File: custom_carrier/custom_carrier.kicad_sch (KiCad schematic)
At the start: 11 parts, among them J1 ERF5-040-05.0-X-DV, J13 PJ-002AH-SMT-TR, J14 87832-1420, J2 ERF5-040-05.0-X-DV, J3 ERF5-040-05.0-X-DV, J4 ERF5-040-05.0-X-DV, J5 45230-220230, J6 45230-220230

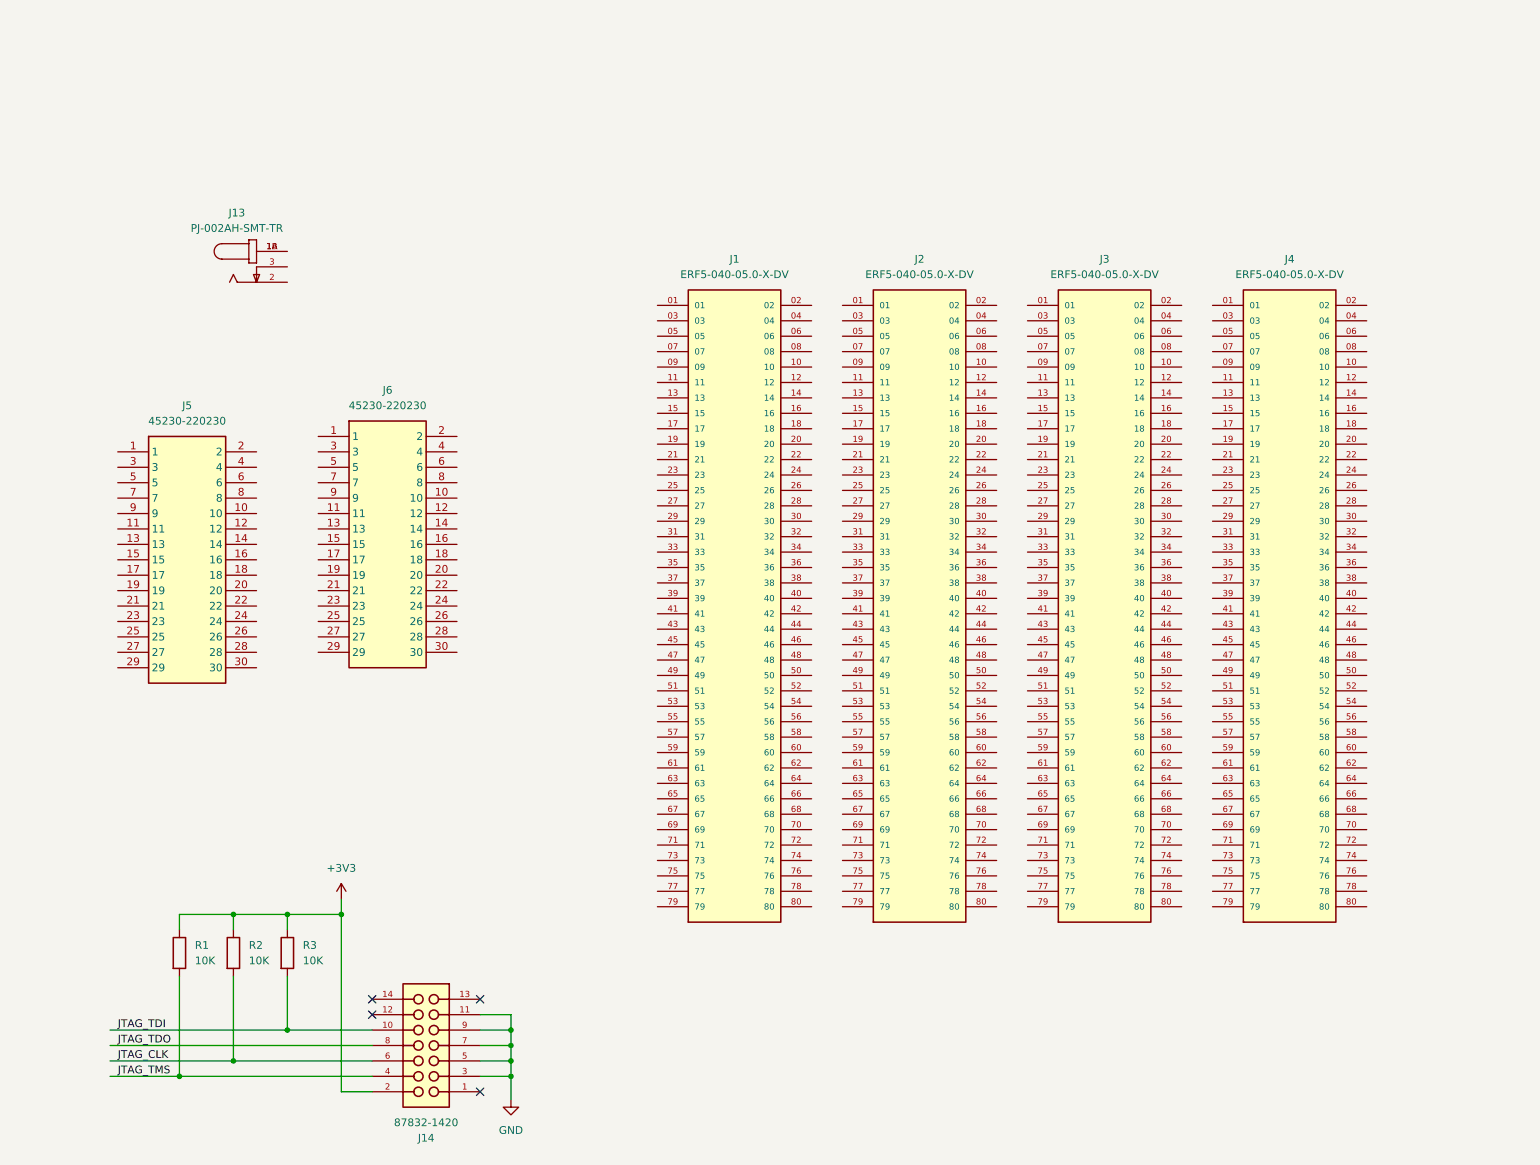
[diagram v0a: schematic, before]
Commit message: working on high-speed cables.
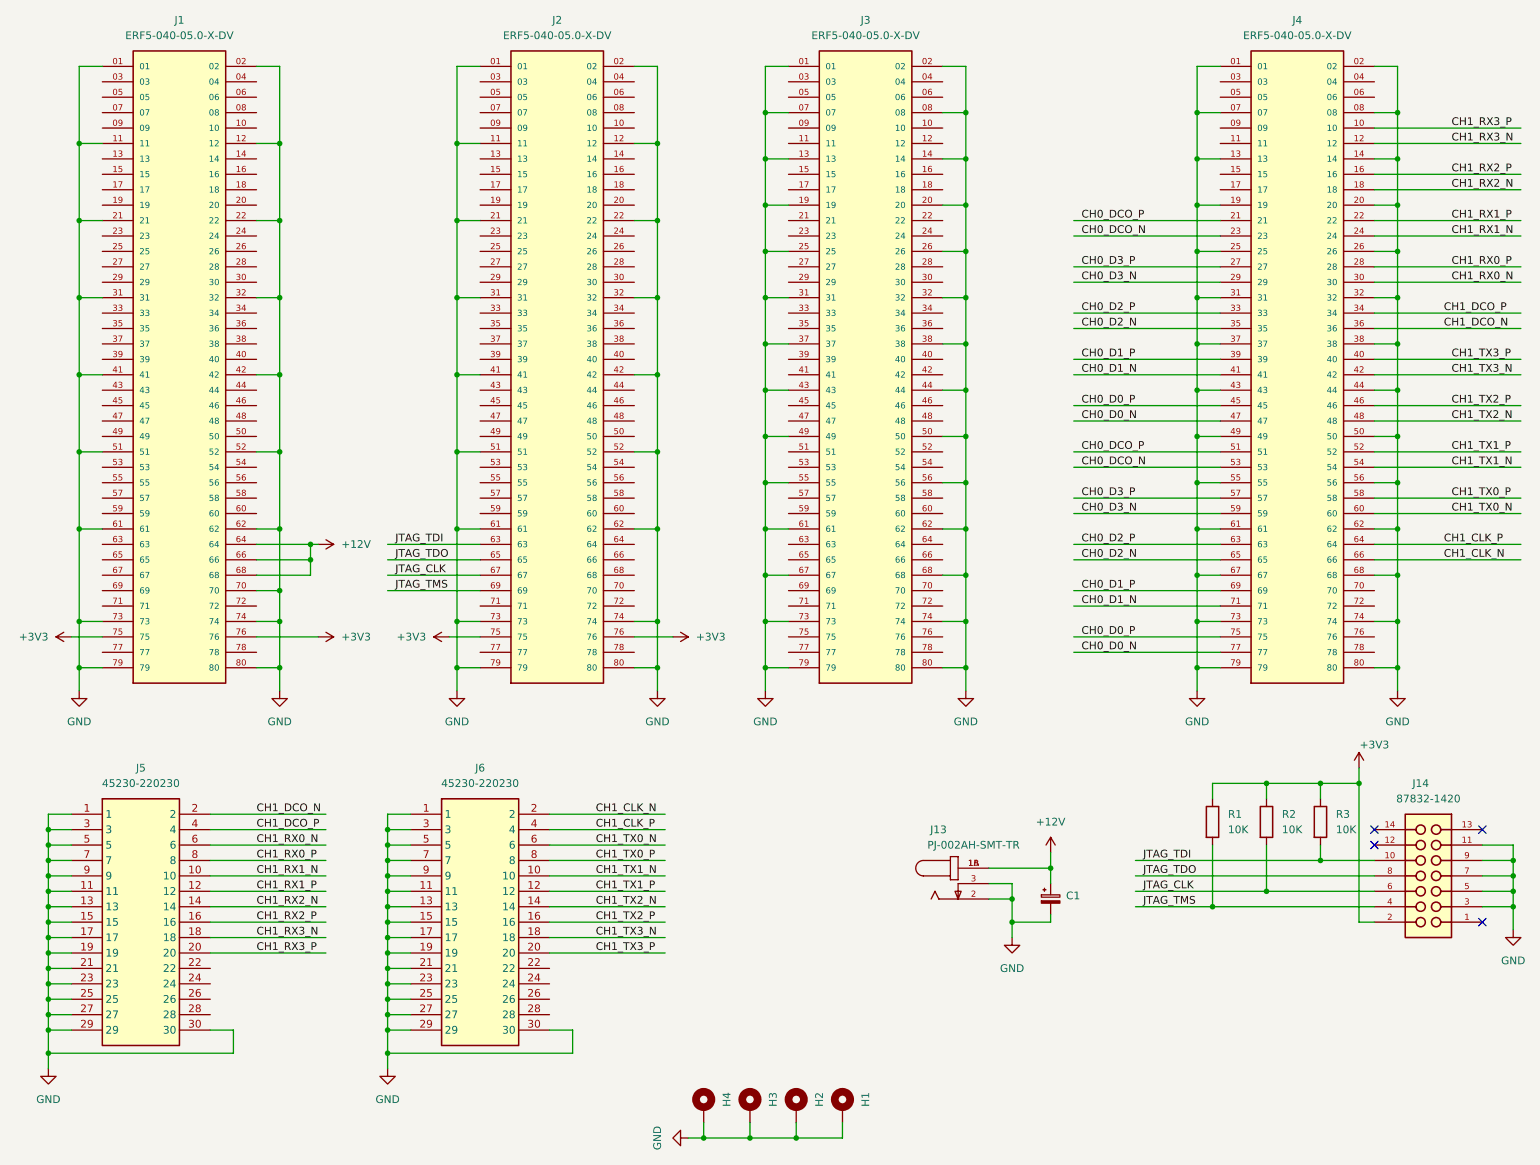
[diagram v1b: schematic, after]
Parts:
- added C1: 22UF/25V, Capacitor_Tantalum_SMD:CP_EIA-3528-15_AVX-H, symbol Device:C_Polarized_Small
- added H1, H2, H3, H4: standoff_hole, MountingHole:MountingHole_2.2mm_M2_DIN965_Pad, symbol pedrolib:standoff_hole
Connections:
- net +3V3: now also J1.75, J1.76, J2.75, J2.76
- net GND: now also J1.01, J1.02, J1.11, J1.12, J1.21, J1.22, J1.31, J1.32, J1.41, J1.42, J1.51, J1.52, J1.61, J1.62, J1.70, J1.73, J1.74, J1.79, J1.80, J13.2, J13.3, J2.01, J2.02, J2.11, J2.12, J2.21, J2.22, J2.31, J2.32, J2.41, J2.42, J2.51, J2.52, J2.61, J2.62, J2.73, J2.74, J2.79, J2.80, J3.01, J3.02, J3.07, J3.08, J3.13, J3.14, J3.19, J3.20, J3.25, J3.26, J3.31, J3.32, J3.37, J3.38, J3.43, J3.44, J3.49, J3.50, J3.55, J3.56, J3.61, J3.62, J3.67, J3.68, J3.73, J3.74, J3.79, J3.80, J4.01, J4.02, J4.07, J4.08, J4.13, J4.14, J4.19, J4.20, J4.25, J4.26, J4.31, J4.32, J4.37, J4.38, J4.43, J4.44, J4.49, J4.50, J4.55, J4.56, J4.61, J4.62, J4.67, J4.68, J4.73, J4.74, J4.79, J4.80, J5.1, J5.11, J5.13, J5.15, J5.17, J5.19, J5.21, J5.23, J5.25, J5.27, J5.29, J5.3, J5.30, J5.5, J5.7, J5.9, J6.1, J6.11, J6.13, J6.15, J6.17, J6.19, J6.21, J6.23, J6.25, J6.27, J6.29, J6.3, J6.30, J6.5, J6.7, J6.9, C1.2, H1.1, H2.1, H3.1, H4.1
- net JTAG_CLK: now also J2.67
- net JTAG_TDI: now also J2.63
- net JTAG_TDO: now also J2.65
- net JTAG_TMS: now also J2.69
- net +12V: now reaches J13.1A, J13.1B
- net +12V: now also J1.64, J1.66, J1.68, C1.1
- net CH1_RX3_P: now reaches J4.10
- net CH1_RX3_P: now also J5.20
- net CH1_RX3_N: now reaches J4.12
- net CH1_RX3_N: now also J5.18
- net CH1_RX2_P: now reaches J4.16
- net CH1_RX2_P: now also J5.16
- net CH1_RX2_N: now reaches J4.18
- net CH1_RX2_N: now also J5.14
- net CH0_DCO_P: now reaches J4.21
- net CH0_DCO_P: now also J4.51
- net CH1_RX1_P: now reaches J4.22
- net CH1_RX1_P: now also J5.12
- net CH0_DCO_N: now reaches J4.23
- net CH0_DCO_N: now also J4.53
- net CH1_RX1_N: now reaches J4.24
- net CH1_RX1_N: now also J5.10
- net CH0_D3_P: now reaches J4.27
- net CH0_D3_P: now also J4.57
- net CH1_RX0_P: now reaches J4.28
- net CH1_RX0_P: now also J5.8
- net CH0_D3_N: now reaches J4.29
- net CH0_D3_N: now also J4.59
- net CH1_RX0_N: now reaches J4.30
- net CH1_RX0_N: now also J5.6
- net CH0_D2_P: now reaches J4.33
- net CH0_D2_P: now also J4.63
- net CH1_DCO_P: now reaches J4.34
- net CH1_DCO_P: now also J5.4
- net CH0_D2_N: now reaches J4.35
- net CH0_D2_N: now also J4.65
- net CH1_DCO_N: now reaches J4.36
- net CH1_DCO_N: now also J5.2
- net CH0_D1_P: now reaches J4.39
- net CH0_D1_P: now also J4.69
- net CH1_TX3_P: now reaches J4.40
- net CH1_TX3_P: now also J6.20
- net CH0_D1_N: now reaches J4.41
- net CH0_D1_N: now also J4.71
- net CH1_TX3_N: now reaches J4.42
- net CH1_TX3_N: now also J6.18
- net CH0_D0_P: now reaches J4.45
- net CH0_D0_P: now also J4.75
- net CH1_TX2_P: now reaches J4.46
- net CH1_TX2_P: now also J6.16
- net CH0_D0_N: now reaches J4.47
- net CH0_D0_N: now also J4.77
- net CH1_TX2_N: now reaches J4.48
- net CH1_TX2_N: now also J6.14
- net CH1_TX1_P: now reaches J4.52
- net CH1_TX1_P: now also J6.12
- net CH1_TX1_N: now reaches J4.54
- net CH1_TX1_N: now also J6.10
- net CH1_TX0_P: now reaches J4.58
- net CH1_TX0_P: now also J6.8
- net CH1_TX0_N: now reaches J4.60
- net CH1_TX0_N: now also J6.6
- net CH1_CLK_P: now reaches J4.64
- net CH1_CLK_P: now also J6.4
- net CH1_CLK_N: now reaches J4.66
- net CH1_CLK_N: now also J6.2
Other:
- title: (none) -> Custom Carrier
- moved on the sheet: J1, J13, J14, J2, J3, J4, J5, J6, R1, R2, R3
